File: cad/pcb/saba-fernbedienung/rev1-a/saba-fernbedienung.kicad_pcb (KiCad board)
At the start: 4 copper layers, 100 x 81.8 mm, 236 parts, among them J201 Conn_ARM_JTAG_SWD_10, J301 Conn_01x04, J302 Conn_01x04, J303 Micro_SD_Card, J304 Conn_01x04, J305 AudioJack3, J306 Conn_01x02, J307 Conn_01x04, J308 Conn_01x01, J309 Conn_01x01, J310 Conn_01x01, J311 Conn_01x04, J312 Conn_01x08, J313 USB_C_Receptacle_USB2.0, K601 G6K-2, K602 G6K-2, K603 G6K-2, K604 G6K-2, K605 G6K-2, K606 G6K-2, K607 EC2-5TNU, Q201 BC856, Q601 BC846, Q602 BC846, Q603 BC846, Q604 BC846, Q605 BC846, Q606 BC846, Q607 BC846, U201 DOIT-DEVKITV1-ESP32-WROOM-32, U301 TSOP31238, U401 TEC2-0911, U402 1117 1.8V, U403 1117 3.3V, U501 ADA4522-2, U502 LM339, U503 LTV-357T, U504 LTV-357T, U505 LTV-357T, U601 LTV-357T, U701 AD8656, U702 VS1053, Y701 12,288MHz

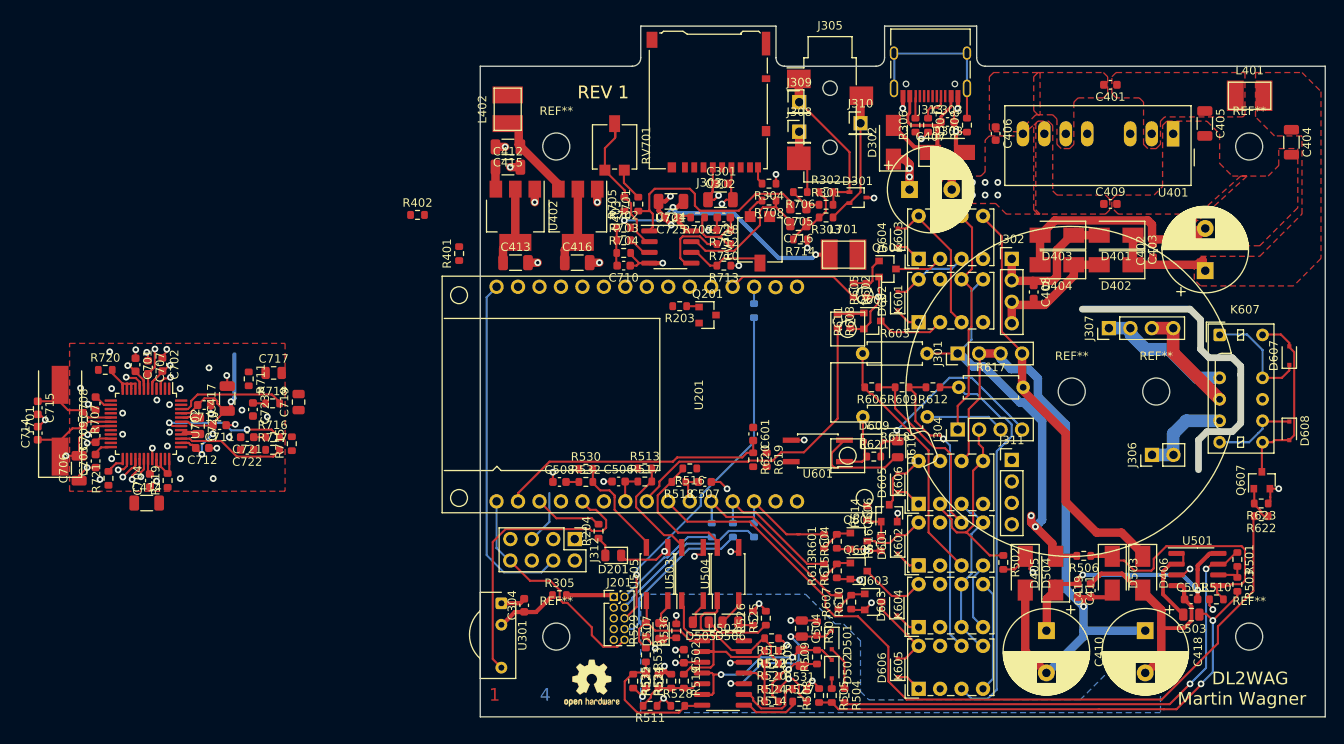
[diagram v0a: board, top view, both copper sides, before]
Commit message: Sicherung
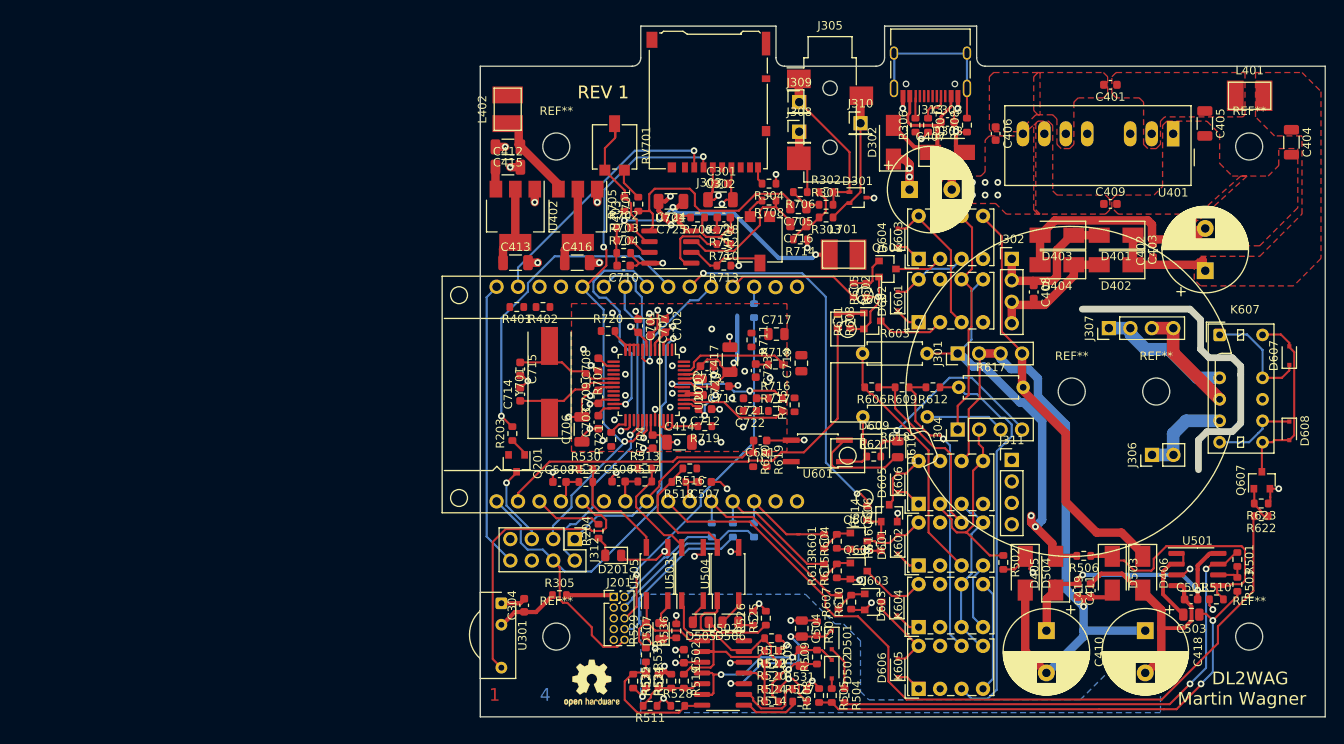
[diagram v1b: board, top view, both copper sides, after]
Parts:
- moved R719 63.9 mm to (126.6, 105.6), turned to 180 degrees
- moved C414 63.5 mm to (123.6, 107.5)
- moved C717 59.7 mm to (135.1, 94.7)
- moved C721 59.7 mm to (131.9, 102.3)
- moved C722 59.7 mm to (131.9, 103.8)
- moved R716 59.7 mm to (134.9, 102.3)
- moved R717 59.7 mm to (134.9, 103.8)
- moved R718 59.7 mm to (134.9, 98.3)
- moved C703 59.7 mm to (114.0, 105.1)
- moved C704 59.7 mm to (120.4, 107.4)
- moved C707 59.7 mm to (120.2, 94.0)
- moved C708 59.7 mm to (114.0, 98.3)
- moved C709 59.7 mm to (114.0, 102.1)
- moved R707 59.7 mm to (112.5, 100.2)
- moved C417 59.7 mm to (129.6, 97.7)
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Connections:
- J312 pad 4: LCD_A0 -> ~RESET
- J312 pad 8: ~RESET -> LCD_A0
- R206 pad 2: SPI_CS_LCD -> SABA_Leise
- U201 pad 23: SABA_Leise -> SPI_CS_LCD
- U201 pad 3: SPI_CS_LCD -> SABA_Leise
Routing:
- net SPI_MOSI: track 2.86 -> 67.3 mm, vias 1 -> 3
- net SABA_Mute: track 0.00 -> 45.0 mm, vias 0 -> 2
- net Net-(R203-Pad2): track 0.00 -> 38.5 mm, vias 0 -> 1
- net SPI_SCK: track 2.84 -> 39.9 mm
- net ~RESET: track 29.3 -> 65.4 mm
- net SPI_CS_SDCARD: track 0.00 -> 30.8 mm, vias 0 -> 1
- net SPI_CS_VS1053: track 0.00 -> 26.4 mm, vias 0 -> 1
- net SPI_MISO: track 2.24 -> 25.8 mm
- net VS1053_DREQ: track 2.62 -> 14.4 mm
- net SPI_CS_LCD: track 2.10 -> 10.2 mm
- net LCD_A0: track 41.6 -> 34.2 mm
- net Net-(C715-Pad1): track 9.02 -> 12.5 mm
- net LCD_BL: track 6.49 -> 9.88 mm, vias 0 -> 1
- net +1V8: track 18.5 -> 21.8 mm, vias 2 -> 3
- net Net-(C714-Pad1): track 9.21 -> 11.8 mm
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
